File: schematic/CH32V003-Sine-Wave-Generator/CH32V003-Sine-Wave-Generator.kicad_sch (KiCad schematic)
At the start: 5 parts, among them U1 CH32V003JxMx, Y1 24MHz

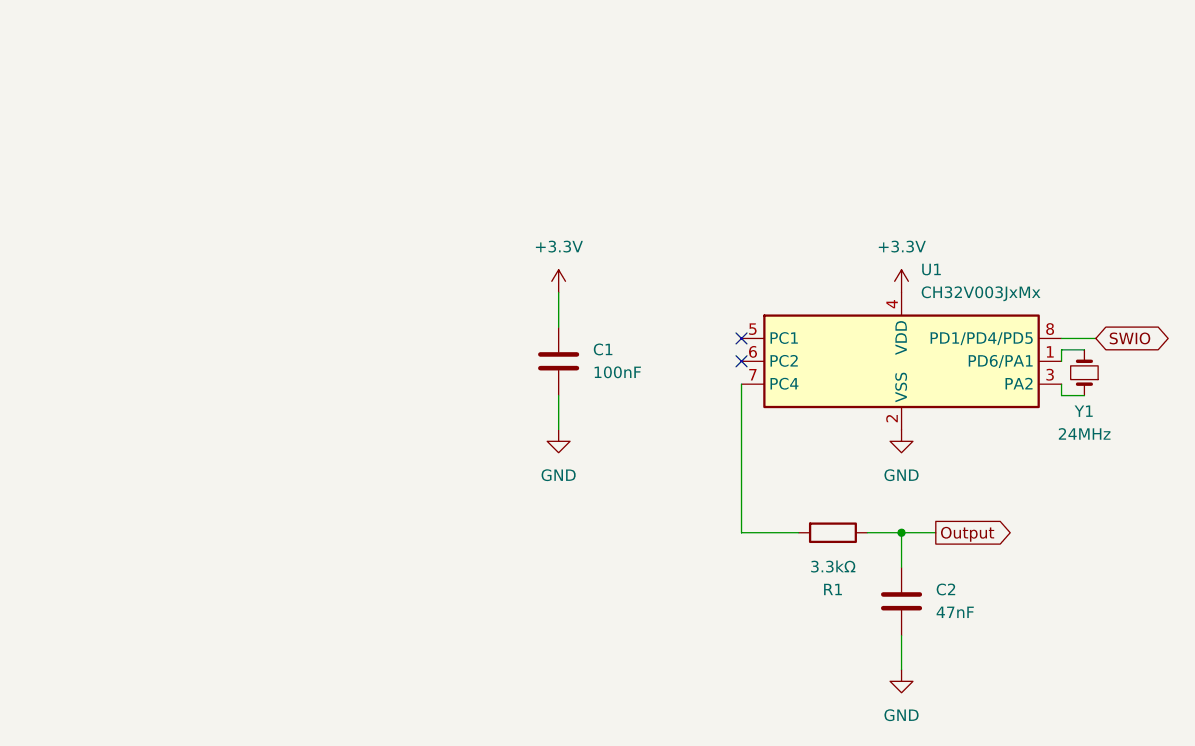
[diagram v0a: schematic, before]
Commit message: Update schematics
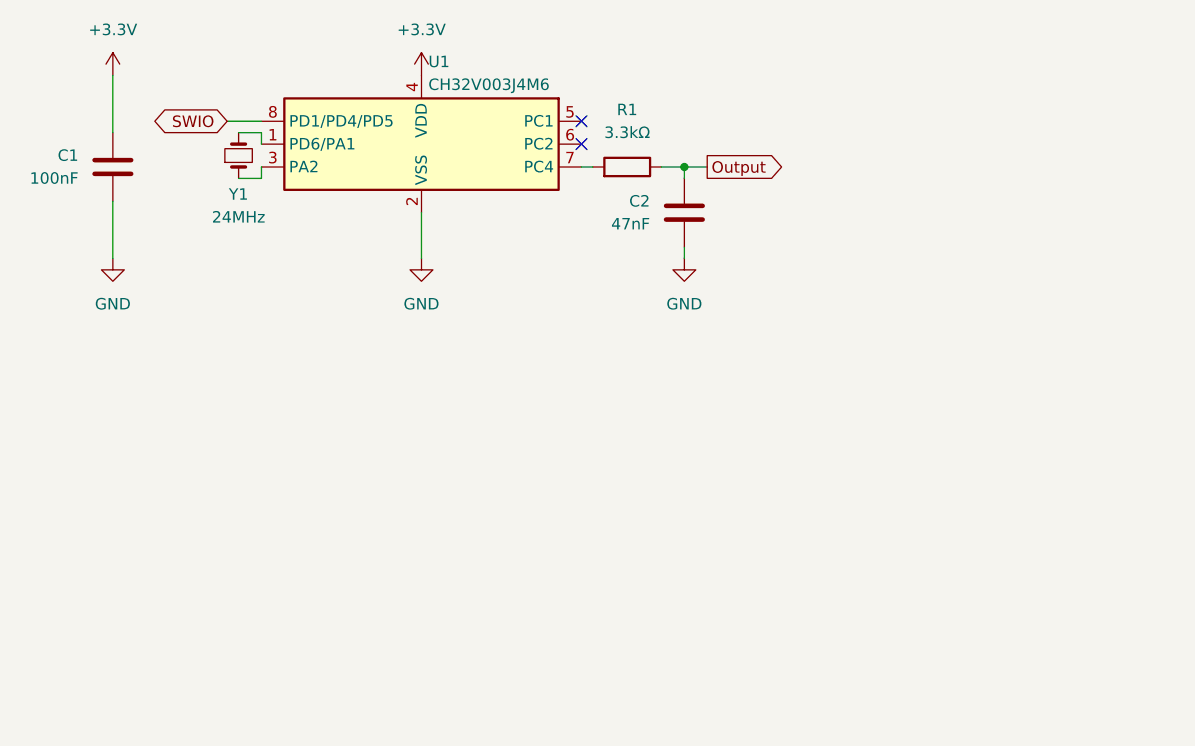
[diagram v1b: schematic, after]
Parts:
- U1: value CH32V003JxMx -> CH32V003J4M6
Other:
- moved on the sheet: C1, C2, R1, U1, Y1
